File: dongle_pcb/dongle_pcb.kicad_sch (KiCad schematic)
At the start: 29 parts, among them J1 USB_A, J2 Conn_01x05_Pin, U1 nRF52840, U2 AP2112K-3.3, U3 2450AT18D0100E

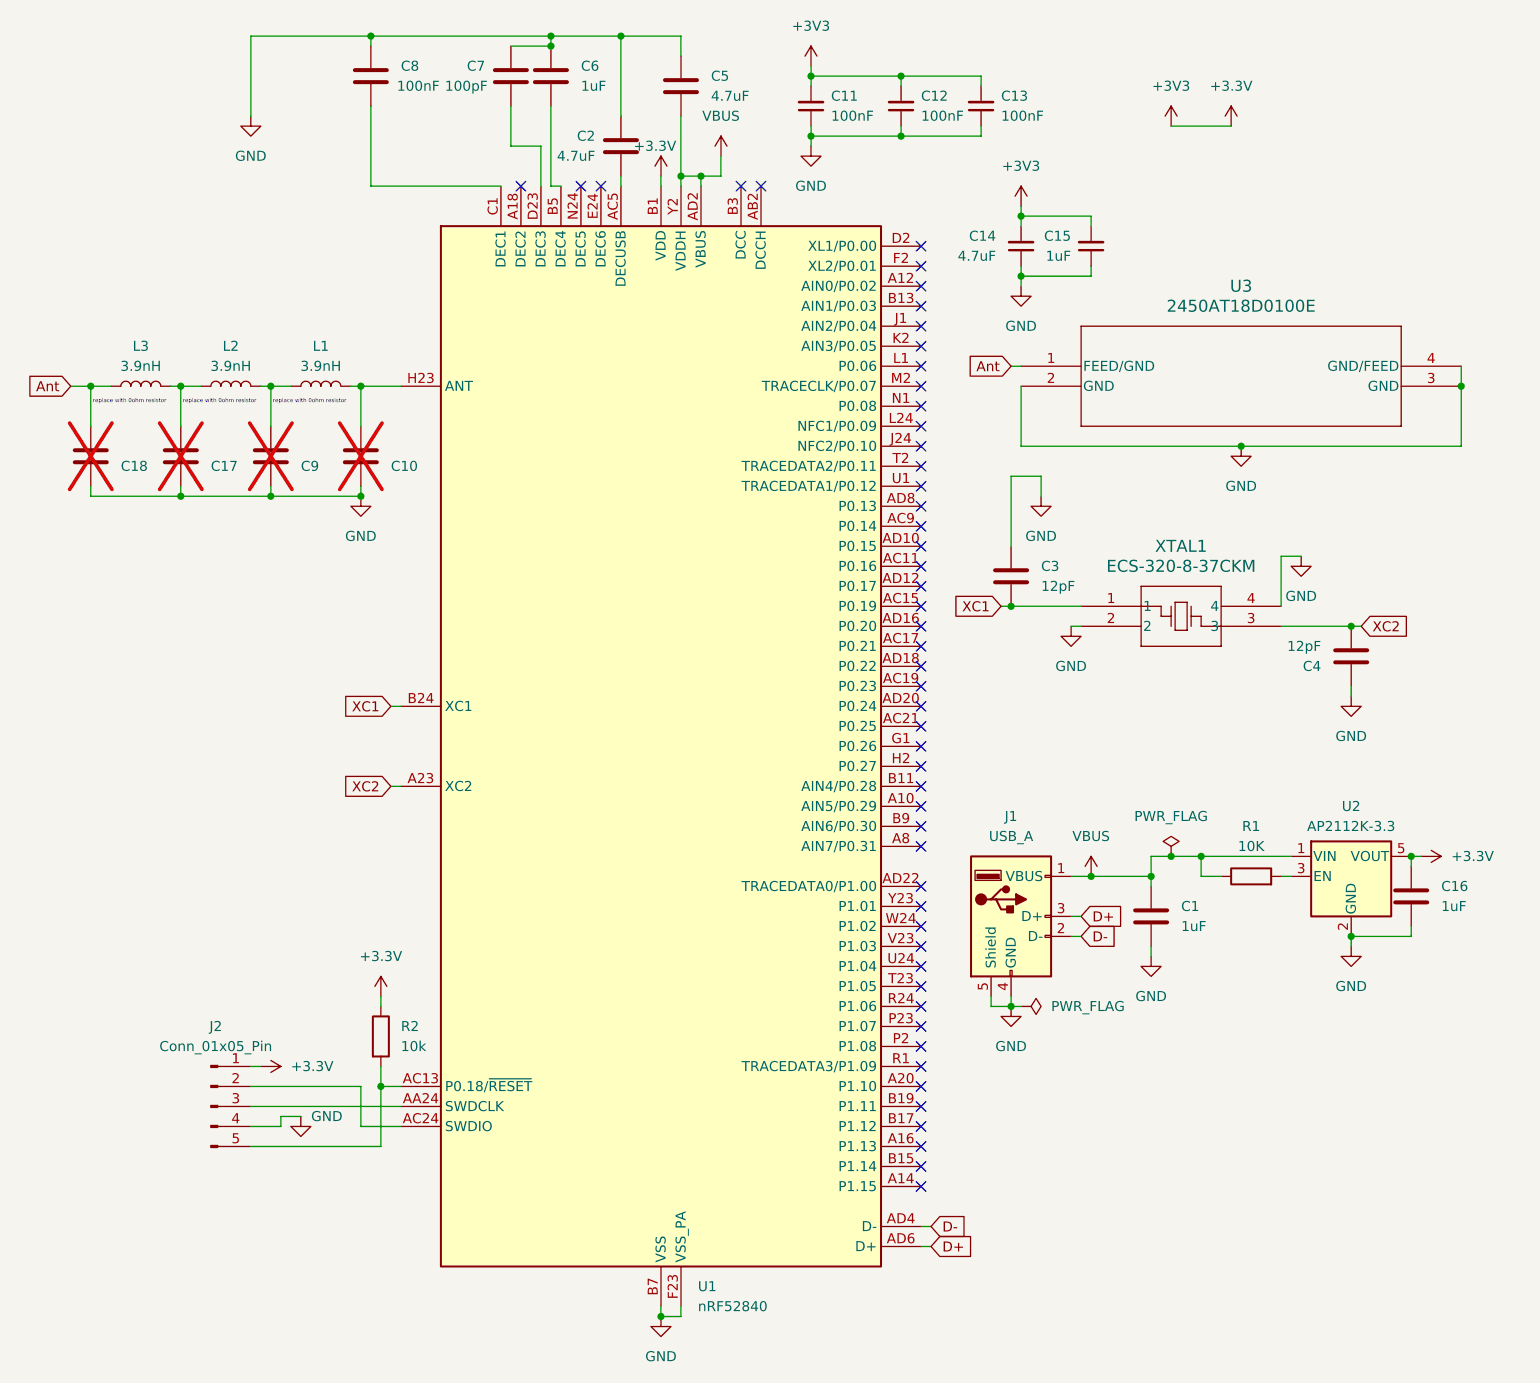
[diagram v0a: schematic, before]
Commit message: restart dongle and finally make ~~america~~ pcbs great again
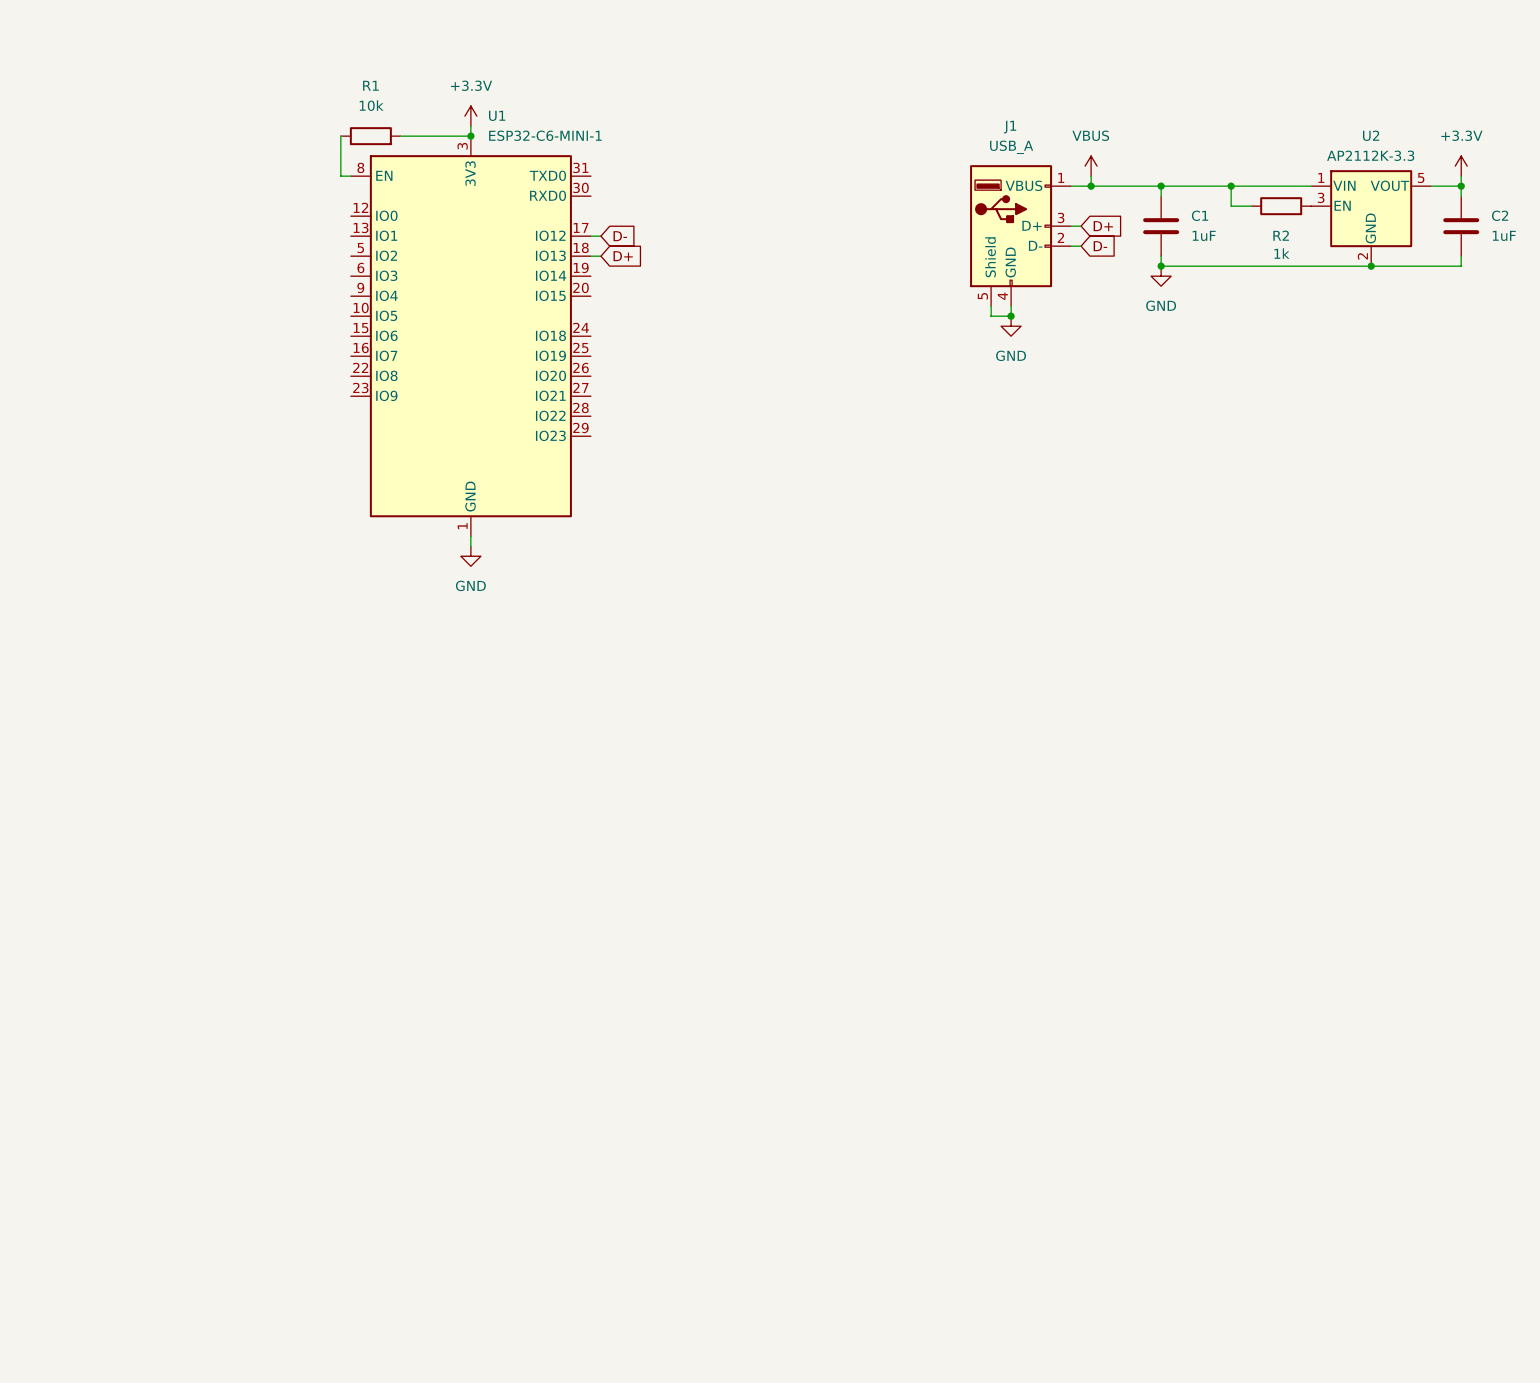
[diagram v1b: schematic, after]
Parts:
- removed C10, C17, C18, C9: ~, Capacitor_SMD:C_0402_1005Metric, symbol Device:C
- removed C11, C12, C13: 100nF, Capacitor_SMD:C_0402_1005Metric, symbol Device:C_Small
- removed C14: 4.7uF, Capacitor_SMD:C_0201_0603Metric, symbol Device:C_Small
- removed C15: 1uF, Capacitor_SMD:C_0603_1608Metric, symbol Device:C_Small
- removed C16, C6: 1uF, Capacitor_SMD:C_0603_1608Metric, symbol Device:C
- removed C3, C4: 12pF, Capacitor_SMD:C_0402_1005Metric, symbol Device:C
- removed C5: 4.7uF, Capacitor_SMD:C_0603_1608Metric, symbol Device:C
- removed C7: 100pF, Capacitor_SMD:C_0402_1005Metric, symbol Device:C
- removed C8: 100nF, Capacitor_SMD:C_0402_1005Metric, symbol Device:C
- removed J2: Conn_01x05_Pin, symbol Connector:Conn_01x05_Pin
- removed L1, L2, L3: 3.9nH, symbol Device:L
- removed U1: nRF52840, Package_DFN_QFN:Nordic_AQFN-73-1EP_7x7mm_P0.5mm, symbol MCU_Nordic:nRF52840
- removed U3: 2450AT18D0100E, RF_Antenna:Johanson_2450AT18x100, symbol Antenna:2450AT18D0100E
- removed XTAL1: ECS-320-8-37CKM, Crystal:Crystal_SMD_2016-4Pin_2.0x1.6mm, symbol Crystal:NX2016AB-32MHZ_ST2
- added U1: ESP32-C6-MINI-1, RF_Module:ESP32-C6-MINI-1, symbol RF_Module:ESP32-C6-MINI-1
- C1: footprint Capacitor_SMD:C_0603_1608Metric -> Capacitor_SMD:C_0603_1608Metric_Pad1.08x0.95mm_HandSolder
- C2: value 4.7uF -> 1uF; footprint Capacitor_SMD:C_0603_1608Metric -> Capacitor_SMD:C_0603_1608Metric_Pad1.08x0.95mm_HandSolder
- J1: footprint (none) -> Connector_USB:USB_A_CNCTech_1001-011-01101_Horizontal
- R1: value 10K -> 10k; footprint (none) -> Capacitor_SMD:C_0603_1608Metric_Pad1.08x0.95mm_HandSolder
- R2: value 10k -> 1k; footprint (none) -> Capacitor_SMD:C_0603_1608Metric_Pad1.08x0.95mm_HandSolder
- U2: footprint Package_TO_SOT_SMD:SOT-23-5 -> Package_TO_SOT_SMD:SOT-23-5_HandSoldering
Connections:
- net +3.3V: now also C2.1, R1.2, U1.3 (3V3); no longer R2.1
- net D+: now also U1.18 (IO13)
- net D-: now also U1.17 (IO12)
- net GND: now also C1.2, C2.2, U1.1 (GND), U1.11 (GND), U1.14 (GND), U1.2 (GND), U1.36 (GND), U1.37 (GND), U1.38 (GND), U1.39 (GND), U1.40 (GND), U1.41 (GND), U1.42 (GND), U1.43 (GND), U1.44 (GND), U1.45 (GND), U1.46 (GND), U1.47 (GND), U1.48 (GND), U1.49 (GND), U1.50 (GND), U1.51 (GND), U1.52 (GND), U1.53 (GND); no longer C2.1
- net VBUS: now also R2.1; no longer R1.1
- net at U2.3 (EN): now also R2.2; no longer R1.2
- new net: R1.1, U1.8 (EN)
- no-connect marks 52 -> 0
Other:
- note removed: "replace with 0ohm resistor"
